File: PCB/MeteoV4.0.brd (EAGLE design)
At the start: 76.2 x 46 mm, 44 parts, among them IC1 MCP73832T, J1 POWER_JACKPTH

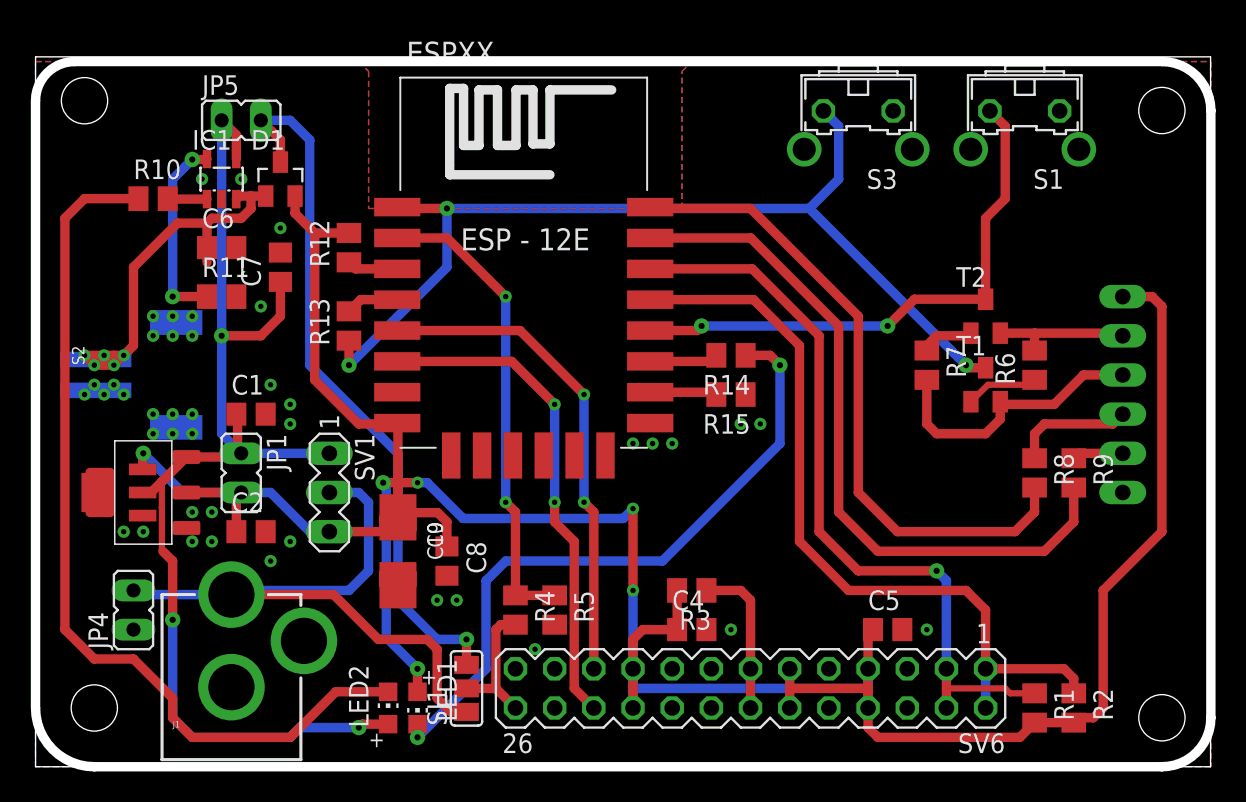
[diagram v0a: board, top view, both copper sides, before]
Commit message: Add files via upload
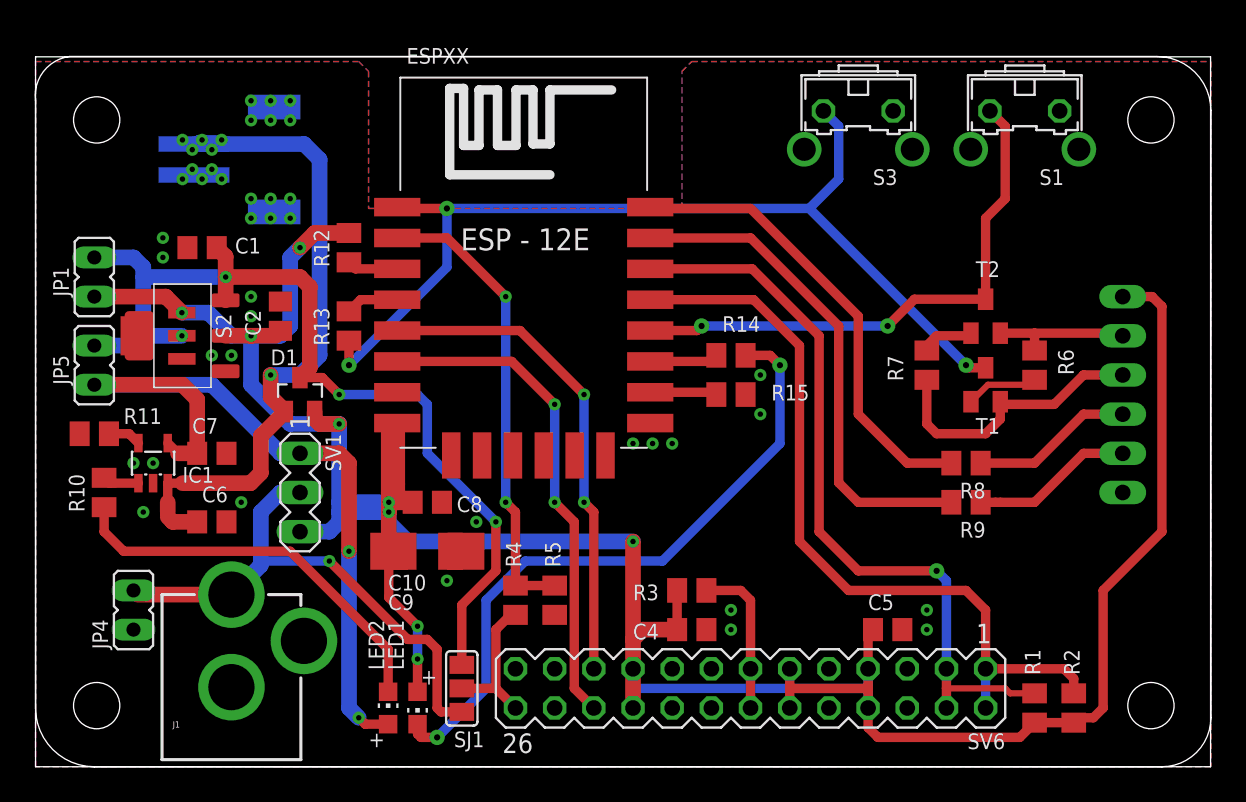
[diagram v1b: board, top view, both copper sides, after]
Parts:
- moved R10 19.3 mm to (4.45, 17.8), turned to 90 degrees
- moved IC1 18.9 mm to (7.62, 19.7)
- moved JP5 18.5 mm to (3.81, 26.0), turned to 0 degrees
- moved C6 17.8 mm to (11.4, 15.9)
- moved JP1 15.9 mm to (3.81, 31.8)
- moved J2 15.3 mm to (14.0, 39.4)
- moved C2 14.1 mm to (15.9, 29.2), turned to 90 degrees
- moved D1 14.0 mm to (17.1, 24.1)
- moved C7 12.9 mm to (11.4, 20.3), turned to 0 degrees
- moved R11 12.1 mm to (3.81, 21.6), turned to 180 degrees
- moved C1 11.3 mm to (10.8, 33.7), turned to 180 degrees
- moved S2 10.5 mm to (9.53, 27.9)
- moved U$1 10.5 mm to (8.89, 27.9)
- moved R9 7.24 mm to (60.3, 17.1), turned to 180 degrees
- moved R8 4.49 mm to (60.3, 19.7), turned to 180 degrees
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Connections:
- net VBAT: now also C1.1, JP1.1, S2.3, U$1.VIN
- net VIN: no longer C1.1, JP1.1, S2.3, U$1.VIN
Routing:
- net N$16: track 57.8 -> 25.9 mm
- net VIN: track 78.0 -> 50.2 mm, vias 3 -> 2
- net N$35: track 26.8 -> 47.4 mm, vias 5 -> 6
- net VBAT: track 46.3 -> 63.3 mm, vias 1 -> 4
- net RXD: track 46.0 -> 32.6 mm
- net TXD: track 42.4 -> 30.1 mm
- net N$5: track 12.6 -> 2.16 mm, vias 2 -> 0
- net VPWR: track 43.5 -> 35.0 mm, vias 0 -> 1
- net VCC: track 191.7 -> 199.3 mm, vias 6 -> 9
- net N$4: track 3.31 -> 10.5 mm
- net N$3: track 7.83 -> 10.5 mm
- net ADC: track 30.8 -> 30.1 mm
- net ANA_IN: track 8.91 -> 9.48 mm
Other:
- board size 76.2 x 46 mm -> 76.2 x 46.1 mm
- board text added: "7/2020"
- board text added: "AIN"
- board text added: "C1"
- board text added: "C10"
- board text added: "C2"
- board text added: "C4"
- board text added: "C5"
- board text added: "C6"
- board text added: "C7"
- board text added: "C8"
- board text added: "C9"
- board text added: "CLK"
- board text added: "D1"
- board text added: "DT"
- board text added: "DTR"
- board text added: "EN/RST"
- board text added: "ESPXX"
- board text added: "GND"
- board text added: "IC1"
- board text added: "IO0"
- board text added: "IO1"
- board text added: "IO2"
- board text added: "J1"
- board text added: "J2"
- board text added: "JP4"
- board text added: "LED1"
- board text added: "LED2"
- board text added: "MeteoV4"
- board text added: "PWR|AIN|VBAT"
- board text added: "R1"
- board text added: "R10"
- board text added: "R11"
- board text added: "R12"
- board text added: "R13"
- board text added: "R14"
- board text added: "R15"
- board text added: "R2"
- board text added: "R3"
- board text added: "R4"
- board text added: "R5"
- board text added: "R6"
- board text added: "R7"
- board text added: "R8"
- board text added: "R9"
- board text added: "RTS"
- board text added: "RXD"
- board text added: "S1"
- board text added: "S2"
- board text added: "S3"
- board text added: "SCL"
- board text added: "SJ1"
- board text added: "SV1"
- board text added: "SV4"
- board text added: "SV6"
- board text added: "T1"
- board text added: "T2"
- board text added: "TXD"
- board text added: "VCC"
- board text added: "VCC-VBAT"
- board text added: "VIN"
- board text added: "VIN-VBAT"
- board text added: "VPWR"
- board text added: "chiptron.cz"
